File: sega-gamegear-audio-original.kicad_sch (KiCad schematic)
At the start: 20 parts, among them CN1 292161-6, CN2 CONN 2P, IC1 TDA2822D, J1 CONN MINI JACK

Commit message: add production files
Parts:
- C1, C2: LCSC Part (none) -> C494824
- C3: LCSC Part (none) -> C178586
- C4, C6, C8: LCSC Part (none) -> C3011705
- C5, C7: LCSC Part (none) -> C336261
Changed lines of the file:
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@@
       (effects (font (size 1.27 1.27)) (justify right))
+    )
+    (property "LCSC Part" "C3011705" (at 182.88 85.09 0)
+      (effects (font (size 1.27 1.27)) hide)
     )
     (pin "1")
@@
       (effects (font (size 1.27 1.27)))
     )
+    (property "LCSC Part" "C336261" (at 161.29 83.82 0)
+      (effects (font (size 1.27 1.27)) hide)
+    )
     (pin "1")
     (pin "2")
@@
       (effects (font (size 1.27 1.27)) (justify right))
     )
+    (property "LCSC Part" "C3011705" (at 215.9 62.23 0)
+      (effects (font (size 1.27 1.27)) hide)
+    )
     (pin "1")
     (pin "2")
@@
     (property "Manufacturer_Part_Number" "GRM188R72A104KA35J" (at 175.26 113.03 90)
       (effects (font (size 1.27 1.27)) (justify right))
+    )
+    (property "LCSC Part" "C3011705" (at 182.88 110.49 0)
+      (effects (font (size 1.27 1.27)) hide)
     )
     (pin "1")
@@
   )
   (symbol (lib_id "EEEFT0J331AP:EEEFT0J331AP") (at 149.86 62.23 270) (unit 1)
-    (in_bom yes) (on_board yes) (dnp no) (fields_autoplaced)
+    (in_bom yes) (on_board yes) (dnp no)
     (property "Reference" "C3" (at 152.4 59.2582 90)
       (effects (font (size 1.27 1.27)) (justify left))
@@
       (effects (font (size 1.27 1.27)) (justify left))
     )
+    (property "LCSC Part" "C178586" (at 146.05 62.23 0)
+      (effects (font (size 1.27 1.27)) hide)
+    )
     (pin "1")
     (pin "2")
@@
       (effects (font (size 1.27 1.27)) (justify left))
     )
+    (property "LCSC Part" "C494824" (at 113.03 90.17 0)
+      (effects (font (size 1.27 1.27)) hide)
+    )
     (pin "1")
     (pin "2")
@@
       (effects (font (size 1.27 1.27)))
     )
+    (property "LCSC Part" "C336261" (at 161.29 109.22 0)
+      (effects (font (size 1.27 1.27)) hide)
+    )
     (pin "1")
     (pin "2")
@@
       (effects (font (size 1.27 1.27)) (justify left))
     )
-    (pin "1")
+    (property "LCSC Part" "C494824" (at 113.03 113.03 0)
+      (effects (font (size 1.27 1.27)) hide)
+    )
+    (pin "1")

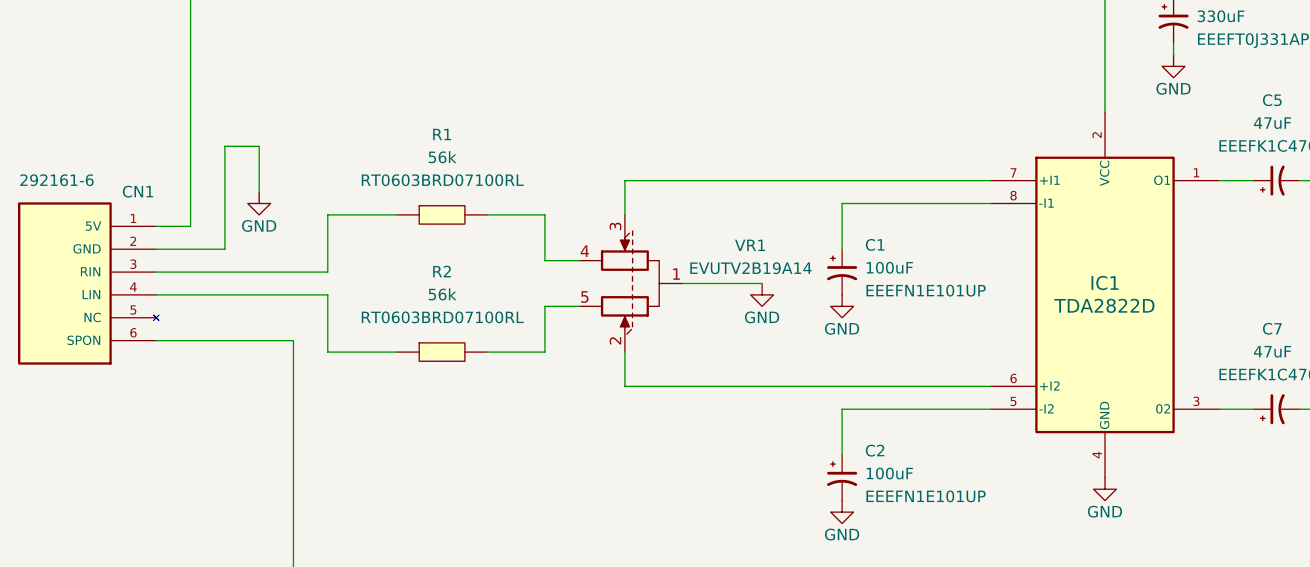
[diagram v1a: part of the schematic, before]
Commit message: update production files
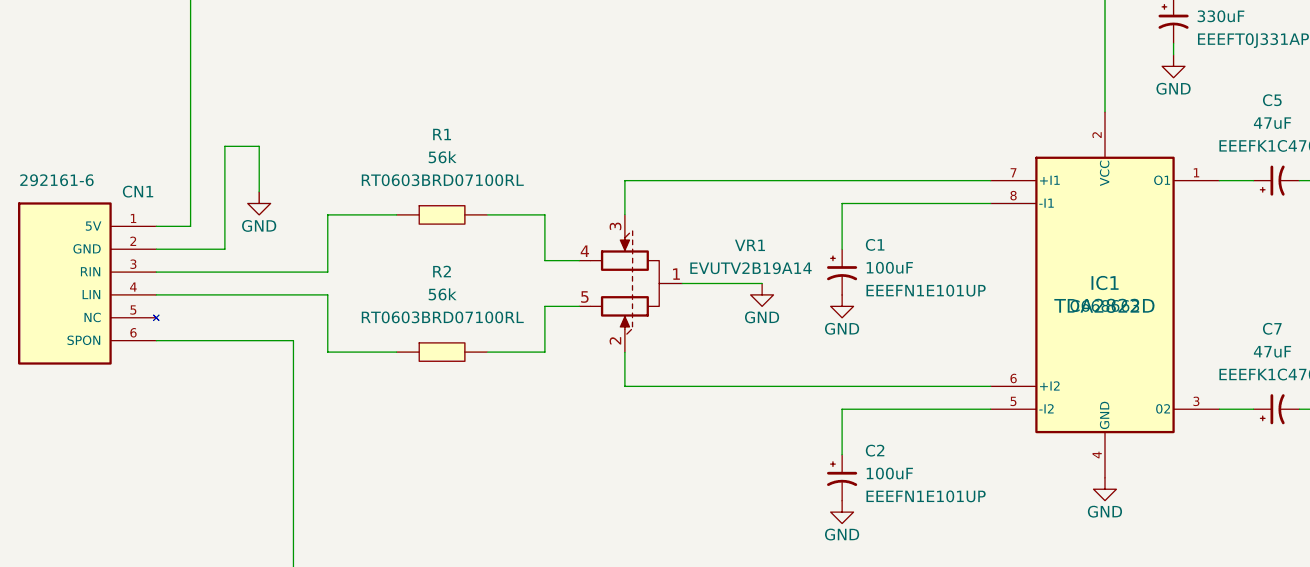
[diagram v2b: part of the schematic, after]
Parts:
- CN1: LCSC Part (none) -> C499123
- CN2: LCSC Part (none) -> C86484
- IC1: LCSC Part (none) -> C668663
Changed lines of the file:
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@@
       (effects (font (size 1.27 1.27)) hide)
+    )
+    (property "LCSC Part" "C668663" (at 142.24 93.98 0)
+      (effects (font (size 1.27 1.27)))
     )
     (pin "4")
@@
       (effects (font (size 1.27 1.27)) hide)
     )
+    (property "LCSC Part" "C499123" (at 26.67 101.6 0)
+      (effects (font (size 1.27 1.27)) hide)
+    )
     (pin "1")
     (pin "2")
@@
       (effects (font (size 1.27 1.27)) (justify left))
     )
-    (pin "1")
+    (property "LCSC Part" "C86484" (at 243.84 134.62 0)
+      (effects (font (size 1.27 1.27)) hide)
+    )
+    (pin "1")
